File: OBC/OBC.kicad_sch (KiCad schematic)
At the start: 10 parts, among them J101 IDC1 (PMS-Raspi), J102 Modo de operación, J103 IDC2 (Raspi-TRU), J104 Conn_01x04, U101 RASPBERRY_PI_ZERO_2_W, U102 BMP280, U103 MPU9250

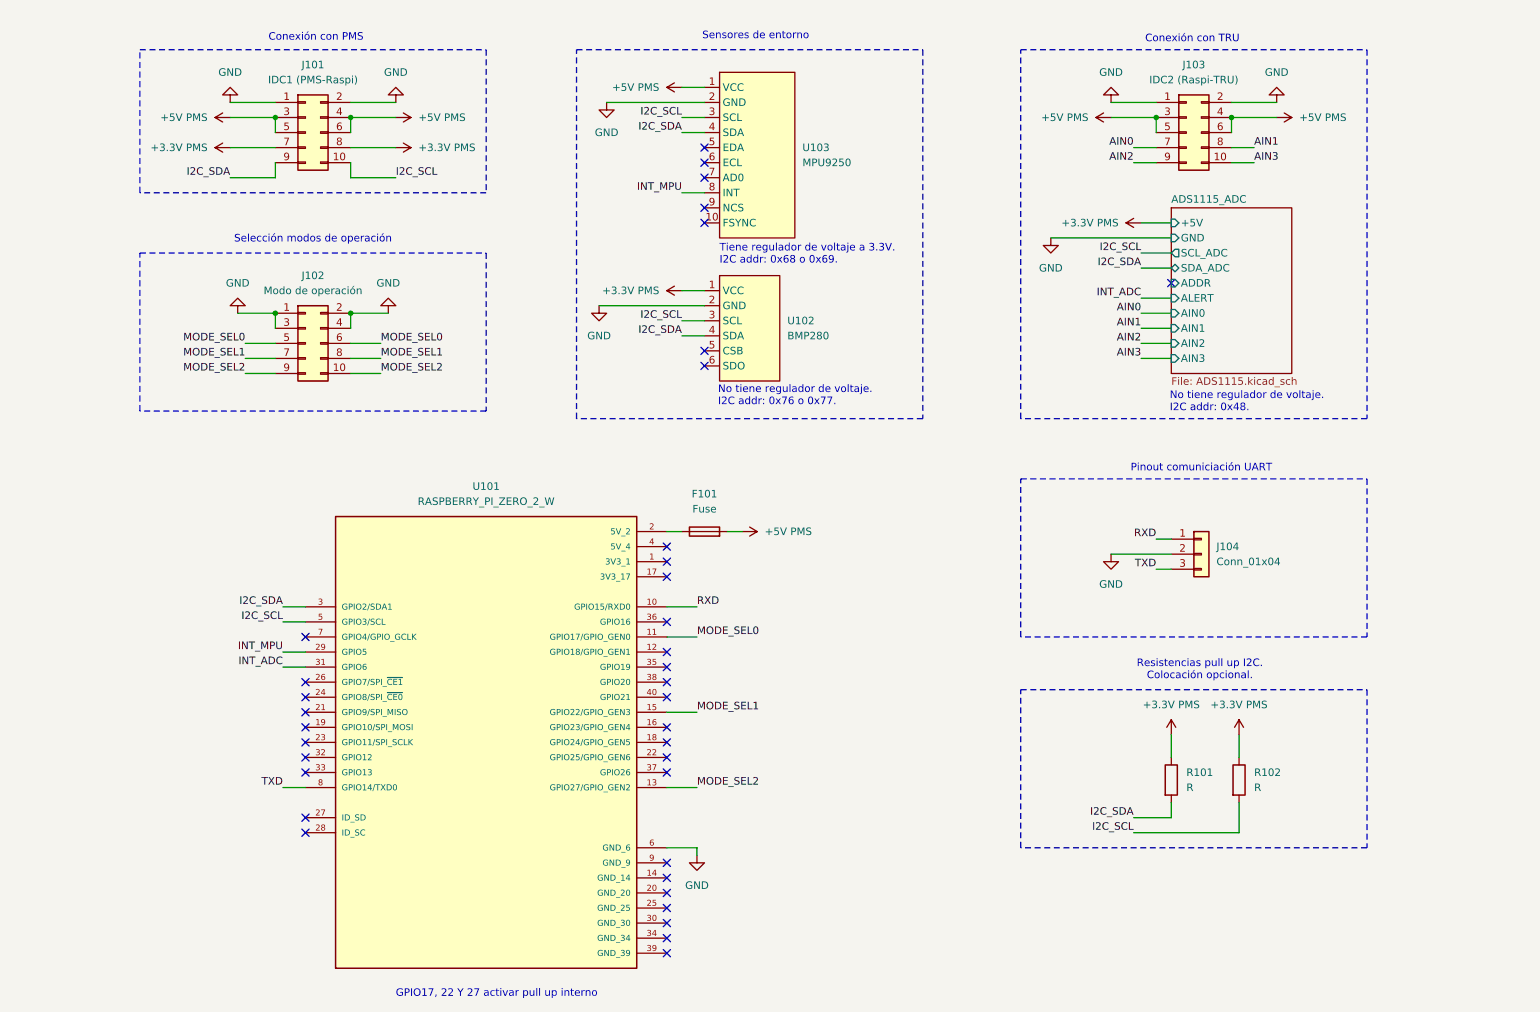
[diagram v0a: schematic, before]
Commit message: Agrega pwr flags
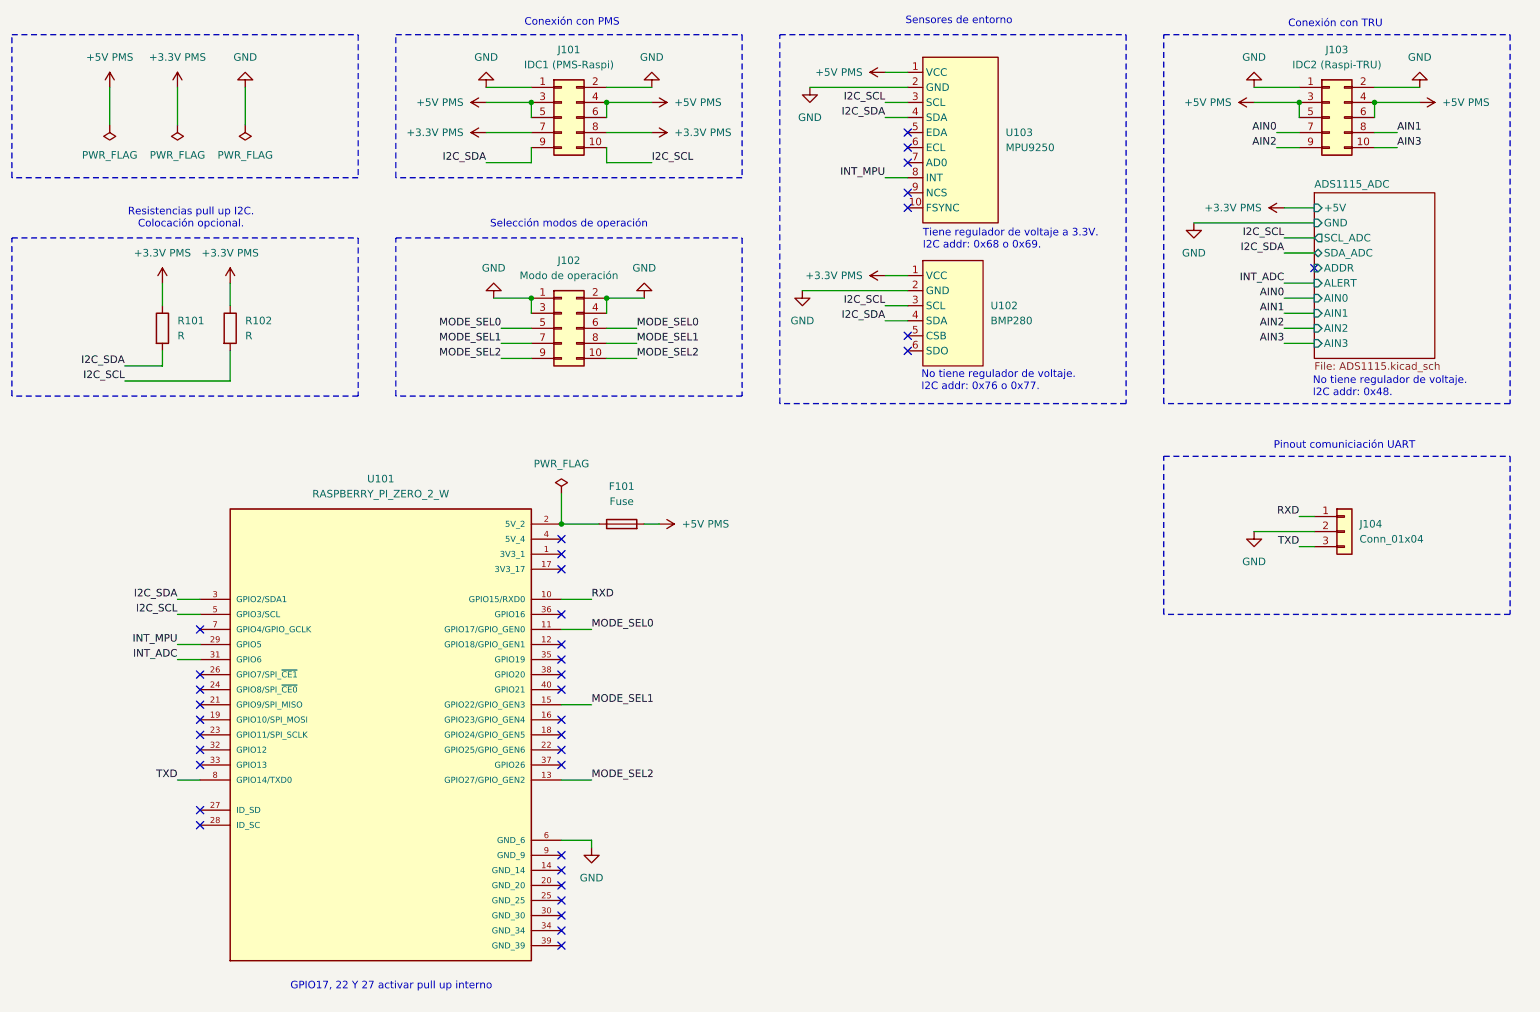
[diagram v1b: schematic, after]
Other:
- moved on the sheet: F101, J101, J102, J103, J104, R101, R102, U101, U102, U103
